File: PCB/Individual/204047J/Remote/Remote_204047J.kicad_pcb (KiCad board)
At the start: 2 copper layers, 170.2 x 116.8 mm, 21 parts, among them J1 Barrel_Jack, J2 Joystick (Servo), SW1 Reset Button, U1 ATmega32-16P, U2 L7809, U3 L7805, U4 L78L33_TO92, U6 NRF24L01, Y1 Crystal

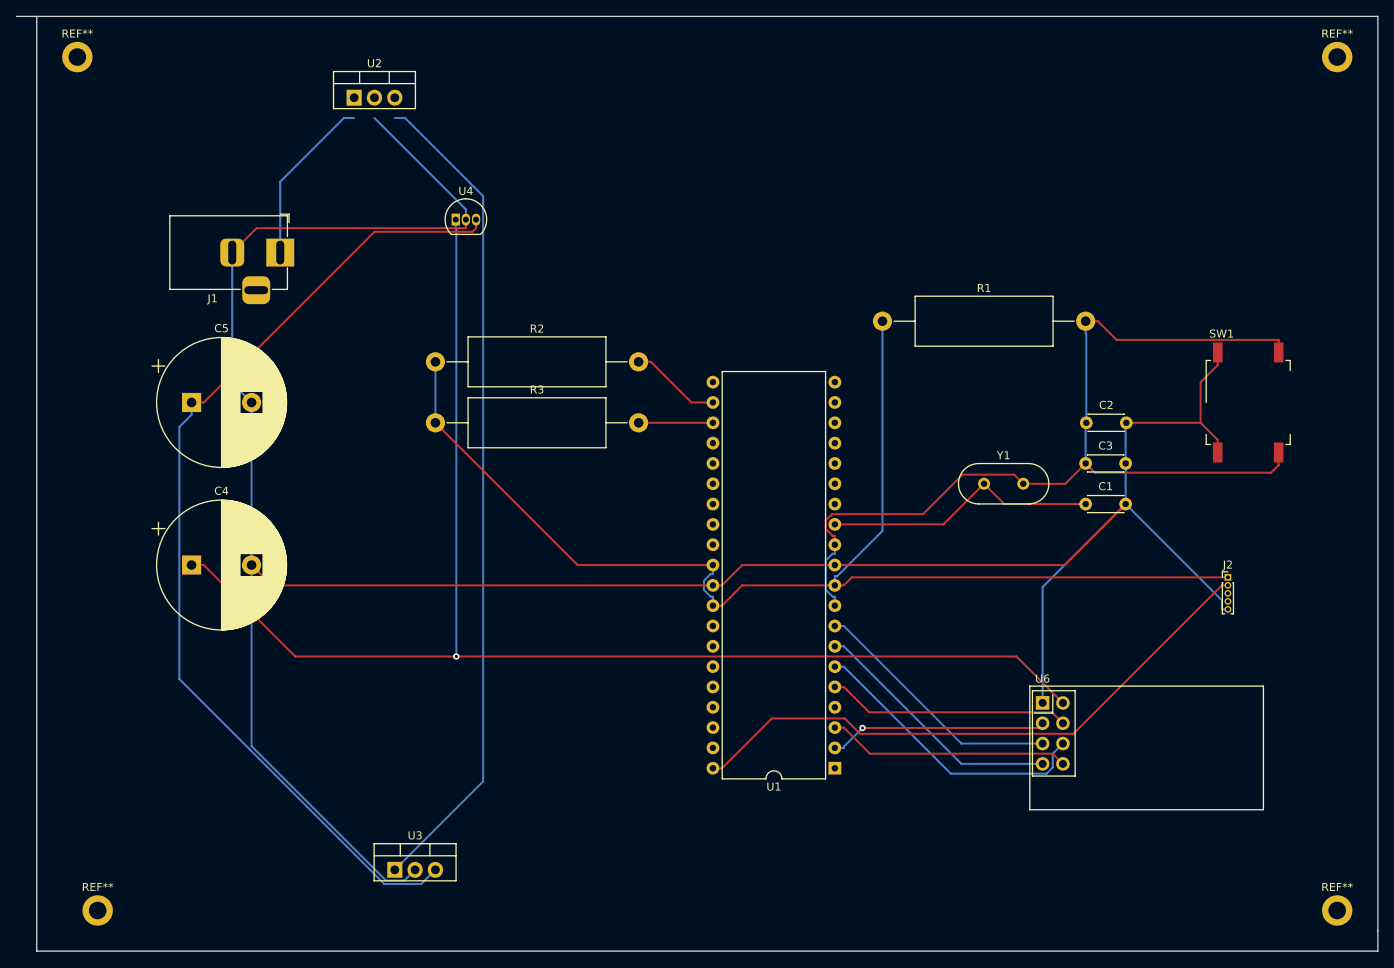
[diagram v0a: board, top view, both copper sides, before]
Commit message: Update Camera Holder PCB 204047J
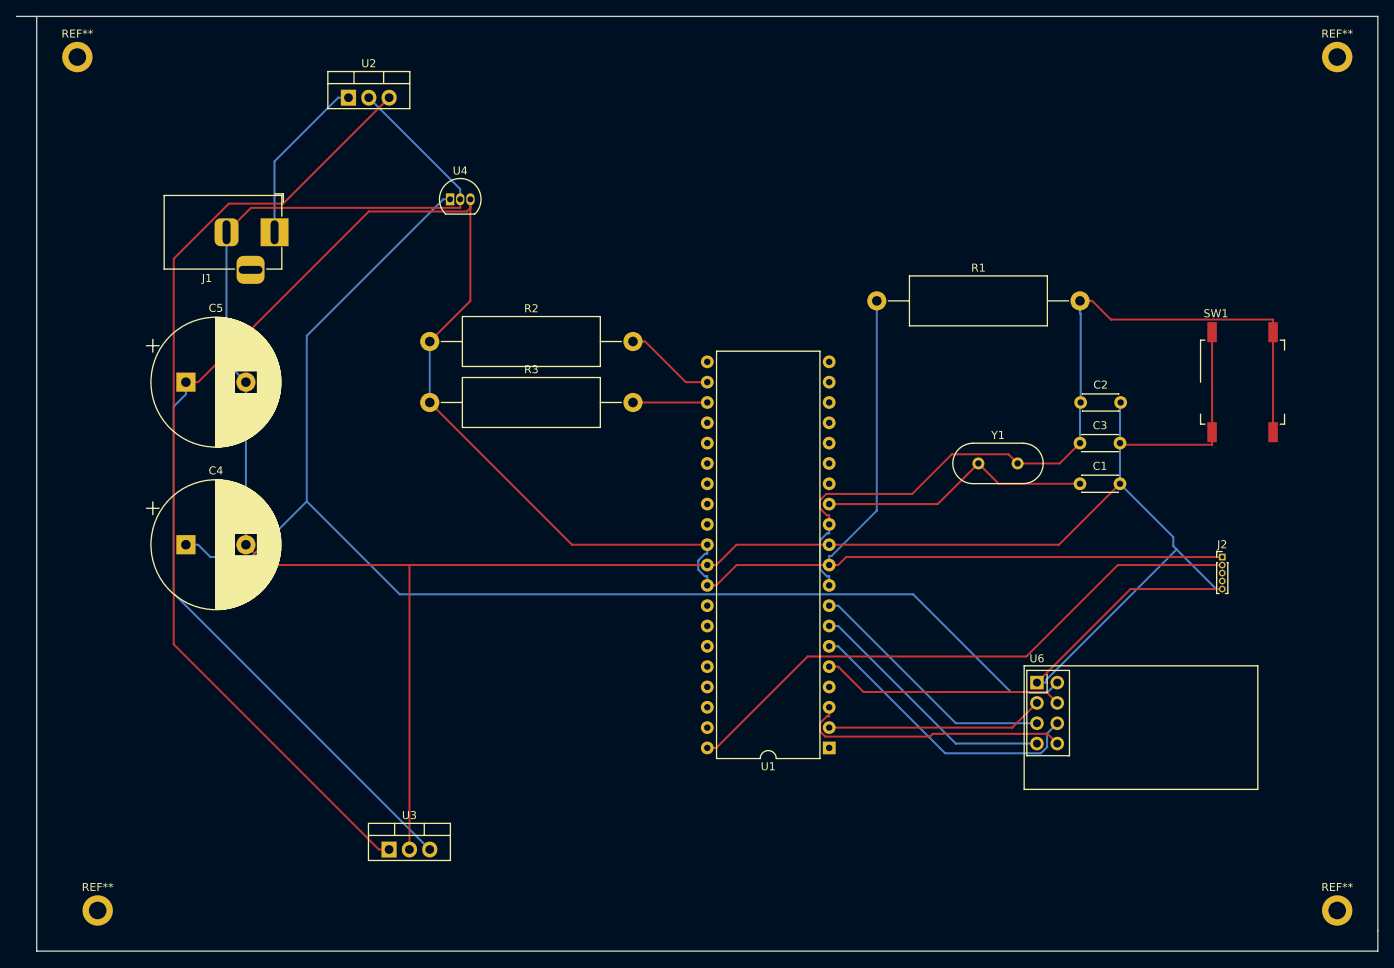
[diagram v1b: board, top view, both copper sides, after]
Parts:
- moved R3 2.64 mm to (112.6, 68.6)
- moved U3 2.64 mm to (107.5, 124.5)
- moved R1 2.64 mm to (168.5, 55.9)
- moved C1 2.64 mm to (193.9, 78.7)
- moved C2 2.64 mm to (194.0, 68.6)
- moved C3 2.64 mm to (193.9, 73.7)
- moved C4 2.64 mm to (82.2, 86.4)
- moved U6 2.64 mm to (188.5, 103.6)
- moved R2 2.64 mm to (112.6, 61.0)
- moved U4 2.64 mm to (115.2, 43.2)
- moved SW1 2.64 mm to (214.2, 66.0)
- moved J1 2.64 mm to (93.2, 47.3)
- moved C5 2.64 mm to (82.2, 66.0)
- moved J2 2.64 mm to (211.7, 87.9)
- moved U1 2.64 mm to (162.6, 111.8)
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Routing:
- net /GND: track 0.00 -> 28.0 mm
- net /Atmega32/GND: track 335.9 -> 318.4 mm
- net Net-(U2-Pad3): track 103.9 -> 121.0 mm
- net Net-(C2-Pad1): track 120.0 -> 106.0 mm
- net /Atmega32/5V: track 281.7 -> 295.4 mm
- net /Atmega32/IRQ: track 30.4 -> 34.2 mm
- net /Power Supply/3.3V: track 170.7 -> 168.5 mm, vias 1 -> 0
- net /Atmega32/A0: track 75.4 -> 73.8 mm
- net /Atmega32/CE: track 27.3 -> 27.2 mm, vias 1 -> 0
